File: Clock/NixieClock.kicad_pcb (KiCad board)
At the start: 2 copper layers, 130.8 x 114.9 mm, 58 parts, among them J1 PJ-079BH, J2 Conn_02x10_Top_Bottom, J3 Conn_02x10_Top_Bottom, J4 Conn_02x10_Top_Bottom, J5 Conn_02x10_Odd_Even, J6 Conn_02x10_Odd_Even, J7 Conn_02x10_Odd_Even, Q1 2N2097, Q2 SI2333DDS-T1-GE3, Q3 T2N7002AK, Q4 2N3906, U1 MC33063AD, U2 HV5622PJ-G, U3 HV5622PJ-G, U4 PHB33NQ20T,118, U5 AP65251, U6 CD40109BPWR, U7 WeMos_mini

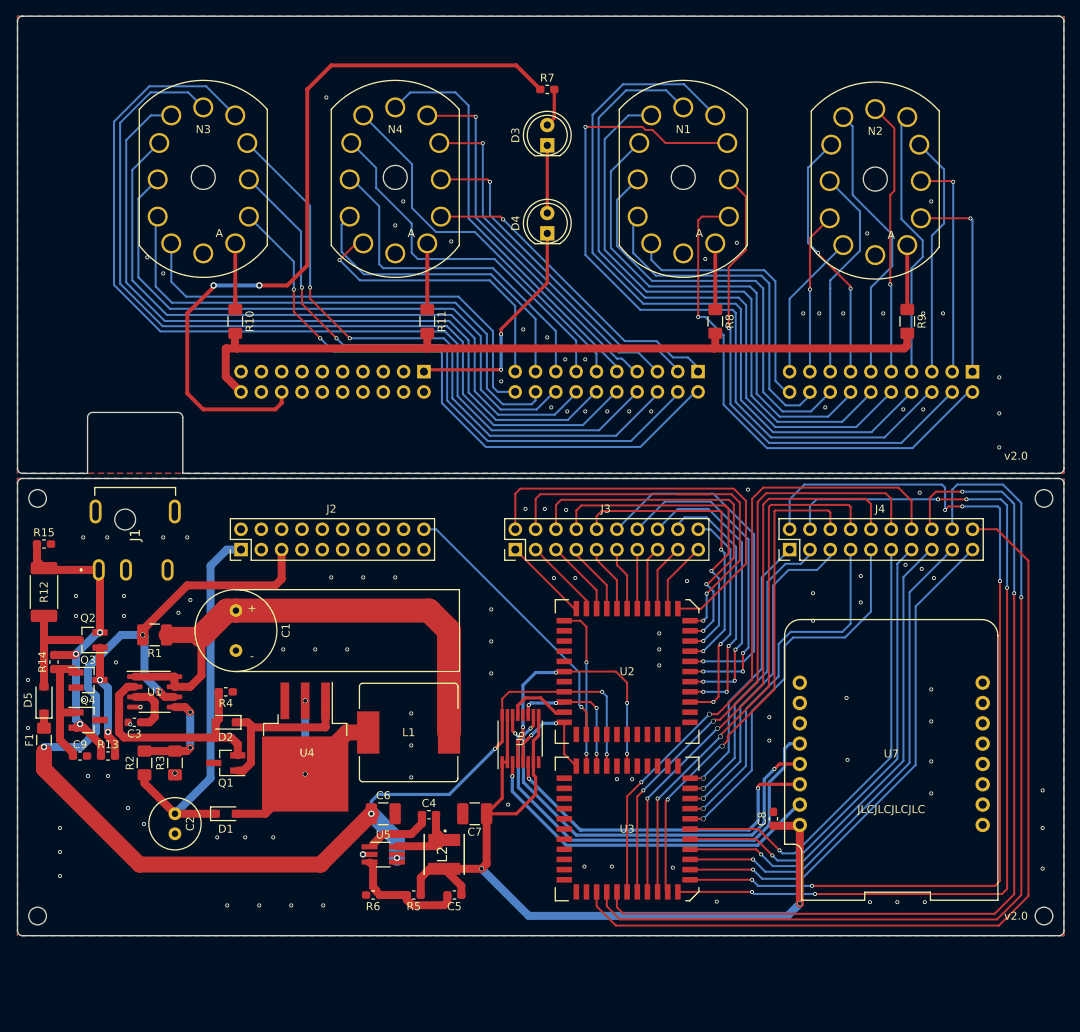
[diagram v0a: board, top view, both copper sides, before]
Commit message: Add v2.0 plots
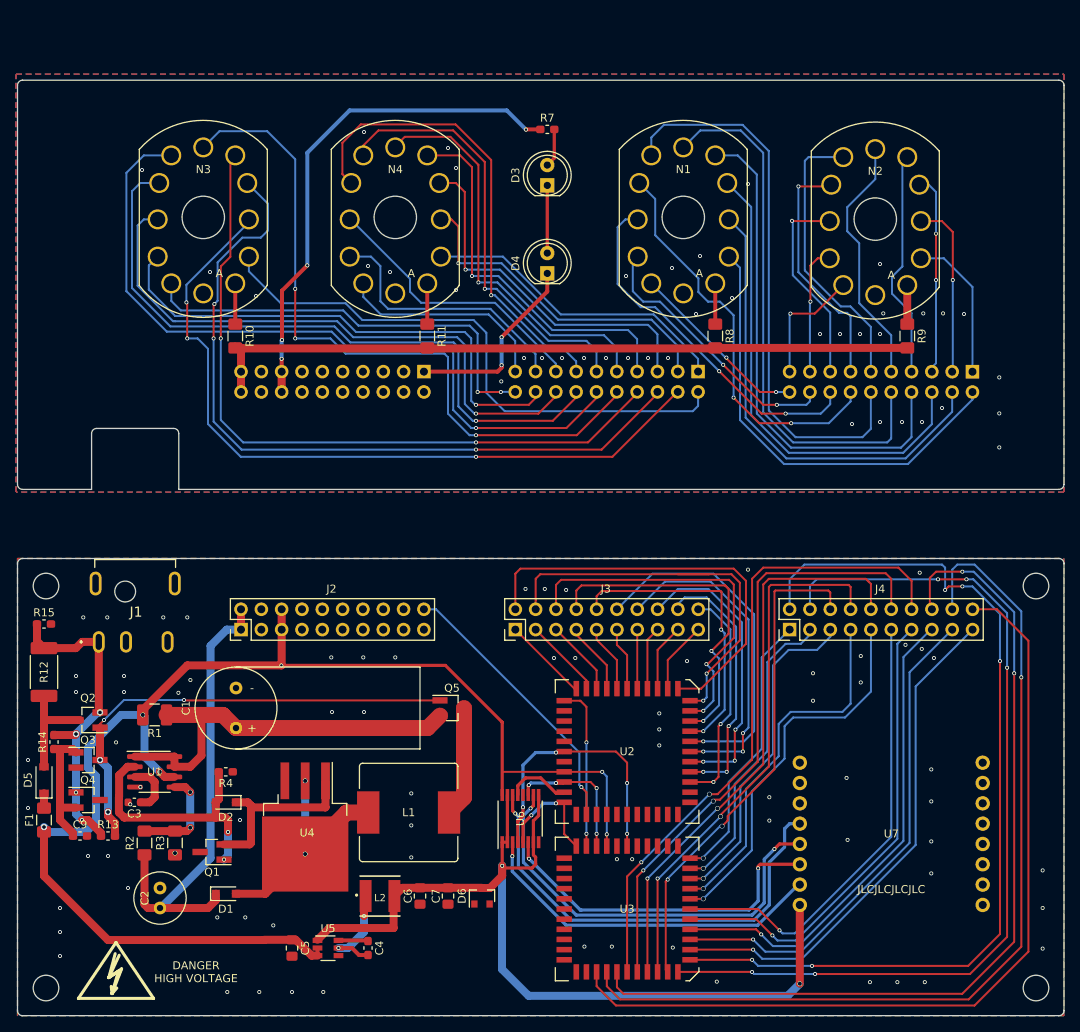
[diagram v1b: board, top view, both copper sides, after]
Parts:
- removed C8: 4.7u, Capacitor_SMD:C_0603_1608Metric_Pad1.05x0.95mm_HandSolder
- removed R5: 115k, Resistor_SMD:R_0603_1608Metric_Pad1.05x0.95mm_HandSolder
- removed R6: 25.5k, Resistor_SMD:R_0603_1608Metric_Pad1.05x0.95mm_HandSolder
- removed the REF** at (164.0, 161.5)
- removed the REF** at (164.0, 109.3)
- removed the REF** at (38.2, 161.5)
- removed the REF** at (38.2, 109.3)
- added D6: BZX84Cxx, Diode_SMD:D_SOT-23_ANK, F.Cu at (93.8, 159.0)
- added Q5: SI2343DS, Package_TO_SOT_SMD:SOT-23_Handsoldering, F.Cu at (90.0, 135.5)
- added REF**: MountingHole_3.2mm_M3, MountingHole:MountingHole_3.2mm_M3, F.Cu at (39.2, 170.5)
- added REF**: MountingHole_3.2mm_M3, MountingHole:MountingHole_3.2mm_M3, F.Cu at (39.2, 120.2)
- added REF**: MountingHole_3.2mm_M3, MountingHole:MountingHole_3.2mm_M3, F.Cu at (163.0, 120.2)
- added REF**: MountingHole_3.2mm_M3, MountingHole:MountingHole_3.2mm_M3, F.Cu at (163.0, 170.5)
- added SYM1: SYM_Flash_Small, Clock:HighVoltage, F.Cu at (48.0, 169.0)
- C1: value 220u -> 330u
- C5: value 33p -> 10u; footprint Capacitor_SMD:C_0603_1608Metric_Pad1.05x0.95mm_HandSolder -> Capacitor_SMD:C_0805_2012Metric_Pad1.15x1.40mm_HandSolder
- C6: value 10u -> 22u; footprint Capacitor_SMD:C_1210_3225Metric_Pad1.42x2.65mm_HandSolder -> Capacitor_SMD:C_0805_2012Metric_Pad1.15x1.40mm_HandSolder
- C7: footprint Capacitor_SMD:C_1210_3225Metric_Pad1.42x2.65mm_HandSolder -> Capacitor_SMD:C_0805_2012Metric_Pad1.15x1.40mm_HandSolder
- Q1: value 2N2097 -> 2N2907
- Q2: value SI2333DDS-T1-GE3 -> SI2343DS
- R10, R11, R8, R9: value 22k -> 33.2k
- R12: value 20 -> 22
- R14: value 115k -> 499k
- R7: value 680 -> 2k
- U5: value AP65251 -> AP63203; footprint Package_TO_SOT_SMD:TSOT-23-6_HandSoldering -> Package_TO_SOT_SMD:TSOT-23-6
- moved C5 21.4 mm to (70.0, 165.5), turned to 270 degrees
- moved C4 18.3 mm to (79.5, 165.5), turned to 270 degrees
- moved C1 14.7 mm to (63.0, 138.0), turned to 90 degrees
- moved U5 13.6 mm to (74.5, 165.5)
- moved C2 11.9 mm to (53.5, 160.5), turned to 90 degrees
- moved Q1 11.3 mm to (60.0, 153.5)
- moved C6 11.3 mm to (86.0, 159.0), turned to 270 degrees
- moved C7 10.8 mm to (89.5, 159.0), turned to 270 degrees
- moved R1 10.0 mm to (52.8, 136.4)
- moved C3 10.0 mm to (50.3, 147.3)
- moved C9 10.0 mm to (43.5, 151.5)
- moved D1 10.0 mm to (61.7, 158.7)
- moved D2 10.0 mm to (61.7, 147.3)
- moved D5 10.0 mm to (39.0, 144.5)
- moved F1 10.0 mm to (39.0, 149.5)
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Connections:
- net Net-(Q2-Pad1) renamed T_ON
- C5 pad 1: +3.3V -> +12V
- C5 pad 2: Net-(C5-Pad2) -> GND
- C6 pad 1: +12V -> +3.3V
- J2 pad 2: Net-(J2-Pad2) -> +170V
- J2 pad 6: Net-(J2-Pad6) -> +12V
- J5 pad 15: Net-(J5-Pad15) -> +12V
- J5 pad 19: Net-(J5-Pad19) -> +170V
- L1 pad 1: Net-(C1-Pad1) -> Net-(L1-Pad1)
- Q1 pad 1: Net-(D2-Pad1) -> Net-(D2-Pad2)
- Q1 pad 2: Net-(D2-Pad2) -> Net-(D2-Pad1)
- Q4 pad 1: Net-(C9-Pad1) -> +12V_UNSAFE
- Q4 pad 2: +12V_UNSAFE -> Net-(C9-Pad1)
- U5 pad 1: Net-(C4-Pad1) -> +3.3V
- U5 pad 2: GND -> +12V
- U5 pad 3: Net-(C5-Pad2) -> +12V
- U5 pad 4: +12V -> GND
- U5 pad 5: +12V -> Net-(C4-Pad2)
- U5 pad 6: Net-(C4-Pad2) -> Net-(C4-Pad1)
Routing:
- net T_ON: track 14.3 -> 58.5 mm, vias 2 -> 4
- net L3_8: track 157.2 -> 121.3 mm, vias 2 -> 1
- net L3_7: track 153.1 -> 122.7 mm
- net L1_7: track 125.0 -> 97.1 mm, vias 0 -> 2
- net +12V: track 262.5 -> 236.0 mm
- net L1_6: track 115.7 -> 96.0 mm, vias 0 -> 3
- net L1_8: track 87.4 -> 103.7 mm, vias 2 -> 3
- net L3_6: track 141.2 -> 125.4 mm
- net L1_9: track 87.3 -> 102.9 mm, vias 2 -> 3
- net Net-(C5-Pad2): track 15.0 -> 0.00 mm
- net Net-(C1-Pad1): track 65.6 -> 50.8 mm
- net Net-(L1-Pad1): track 0.00 -> 13.8 mm
- net L2_4: track 88.3 -> 101.5 mm, vias 2 -> 3
- net L3_4: track 107.5 -> 96.3 mm, vias 1 -> 3
- net L3_1: track 68.2 -> 57.7 mm, vias 1 -> 3
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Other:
- board size 130.8 x 114.9 mm -> 130.8 x 116.9 mm
- board text added: "DANGER HIGH VOLTAGE"
- board text removed: "v2.0"
